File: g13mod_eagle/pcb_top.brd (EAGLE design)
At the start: 85.2 x 17.3 mm, 4 parts

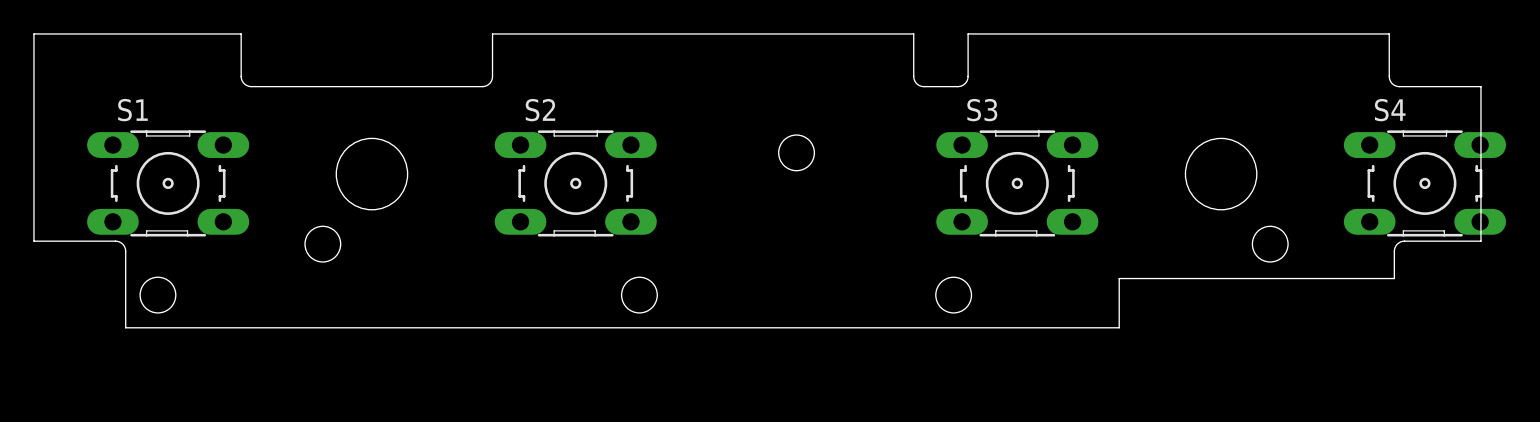
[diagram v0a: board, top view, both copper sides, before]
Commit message: wiring
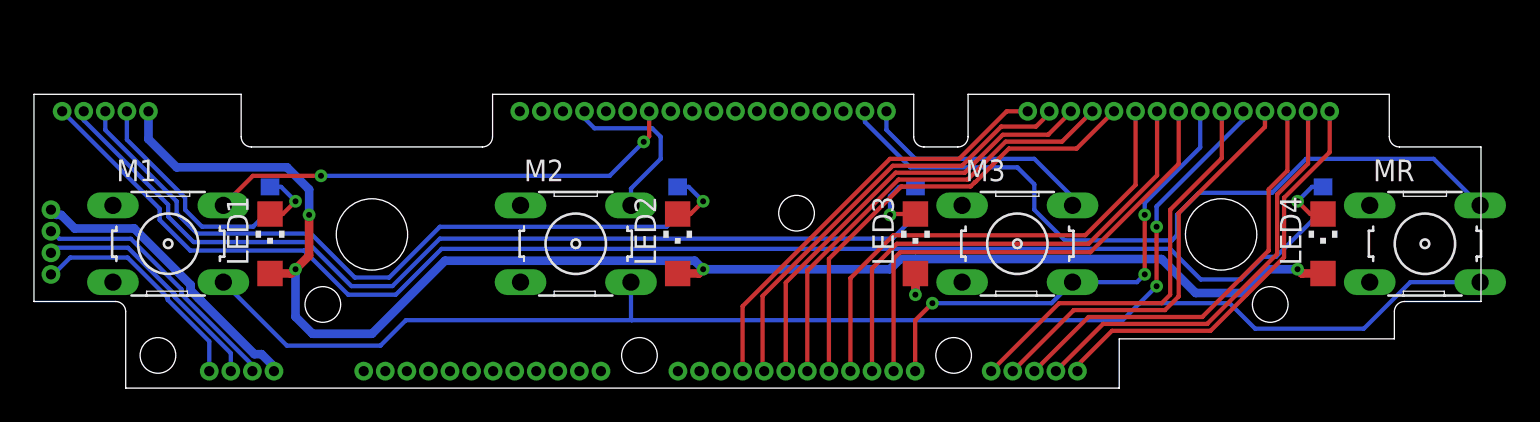
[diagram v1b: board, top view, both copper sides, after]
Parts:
- removed S1, S2, S3, S4: (no value), switch-omron:B3F-10XX
- added CN6: (no value), pinhead-half-pitch:THROUHOLE18
- added CN7: (no value), pinhead-half-pitch:THROUHOLE15
- added JP2, JP3: (no value), pinhead-half-pitch:THROUHOLE05
- added JP4, JP7: (no value), pinhead-half-pitch:THROUHOLE04
- added JP5, JP6: (no value), pinhead-half-pitch:THROUHOLE12
- added LED1, LED2, LED3, LED4: (no value), led:CHIPLED_1206
- added M1, M2, M3, MR: (no value), switch-omron:B3F-10XX
- added R1, R2, R3, R4: (no value), rcl:R0603
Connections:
- new net CN6_1: CN6.1, M3.2
- new net CN6_10: CN6.10, JP5.5
- new net CN6_11: CN6.11, JP5.6
- new net CN6_12: CN6.12, M1.2
- new net CN6_13: CN6.13, JP5.7
- new net CN6_14: CN6.14, JP5.8
- new net CN6_15: CN6.15, JP5.9, M2.2
- new net CN6_16: CN6.16, JP5.10
- new net CN6_17: CN6.17, JP5.11
- new net CN6_18: CN6.18, JP5.12
- new net CN6_2: CN6.2, MR.2
- new net CN6_3: CN6.3, JP6.10
- new net CN6_4: CN6.4, JP6.11
- new net CN6_5: CN6.5, JP6.12
- new net CN6_6: CN6.6, JP5.1
- new net CN6_7: CN6.7, JP5.2
- new net CN6_8: CN6.8, JP5.3
- new net CN6_9: CN6.9, JP5.4
- new net CN7_1: CN7.1, JP2.1
- new net CN7_10: CN7.10, JP6.4
- new net CN7_11: CN7.11, JP6.5
- new net CN7_12: CN7.12, JP6.6
- new net CN7_13: CN7.13, JP6.7
- new net CN7_14: CN7.14, JP6.8
- new net CN7_15: CN7.15, JP6.9
- new net CN7_2: CN7.2, JP2.2
- new net CN7_3: CN7.3, JP2.3
- new net CN7_4: CN7.4, JP2.4
- new net CN7_5: CN7.5, M1.4, M2.4, MR.4
- new net CN7_6: CN7.6, JP2.5
- new net CN7_7: CN7.7, JP6.1, M3.4
- new net CN7_8: CN7.8, JP6.2
- new net CN7_9: CN7.9, JP6.3
- new net LED_M1: JP3.4, R1.1
- new net LED_M2: JP3.3, R2.1
- new net LED_M3: JP3.2, R3.1
- new net LED_MR: JP3.1, R4.1
- new net N$1: JP4.1, JP7.1
- new net N$2: JP4.2, JP7.2
- new net N$3: JP4.3, JP7.3
- new net N$4: JP4.4, JP7.4
- new net N$5: JP3.5, LED1.A, LED2.A, LED3.A, LED4.A
- new net N$6: LED1.C, R1.2
- new net N$7: LED2.C, R2.2
- new net N$8: LED3.C, R3.2
- new net N$9: LED4.C, R4.2
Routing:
- net CN7_5: track 0.00 -> 94.5 mm, vias 0 -> 2
- net N$5: track 0.00 -> 91.4 mm, vias 0 -> 5
- net LED_MR: track 0.00 -> 82.5 mm
- net LED_M3: track 0.00 -> 55.7 mm
- net CN6_2: track 0.00 -> 44.4 mm
- net LED_M2: track 0.00 -> 40.3 mm
- net CN7_10: track 0.00 -> 28.9 mm
- net CN7_9: track 0.00 -> 28.9 mm
- net CN7_8: track 0.00 -> 28.8 mm
- net CN7_7: track 0.00 -> 28.6 mm, vias 0 -> 3
- net CN6_12: track 0.00 -> 28.2 mm, vias 0 -> 2
- net CN7_11: track 0.00 -> 27.0 mm
- net CN7_12: track 0.00 -> 26.6 mm
- net CN7_13: track 0.00 -> 26.2 mm
- net CN7_14: track 0.00 -> 25.9 mm
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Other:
- outline, holes or cut-outs redrawn
